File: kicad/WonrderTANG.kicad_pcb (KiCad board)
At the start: 2 copper layers, 101.6 x 90.2 mm, 29 parts, among them CON1 MSX-CONNECTOR, J1 Conn_02x01, J2 AudioJack3, J3 Conn_02x01, Q1 2N3904, U1 SN74LVC245AN, U2 SN74LVC245AN, U3 SN74LVC245AN, U4 SN74LVC245AN, U5 Tang_Nano_20k, U6 SN74LVC245AN

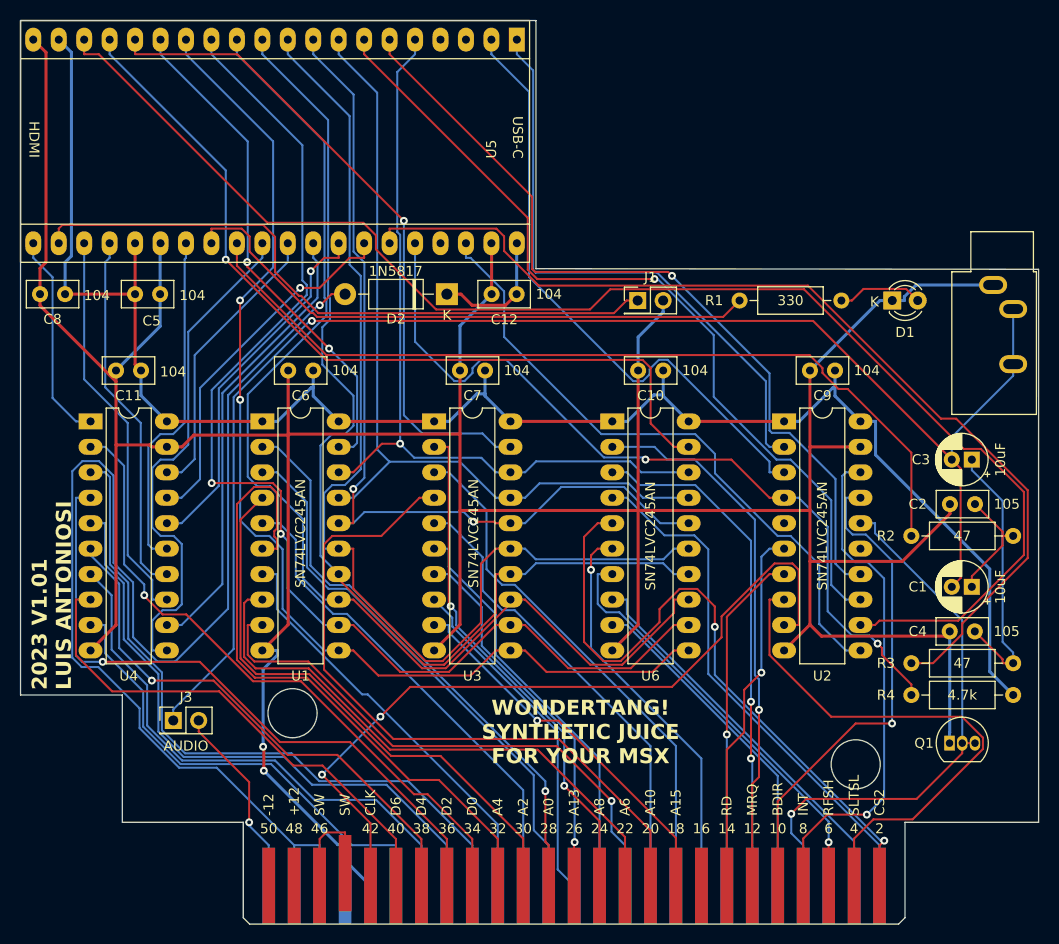
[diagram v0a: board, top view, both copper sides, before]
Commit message: kicad final version 1.01
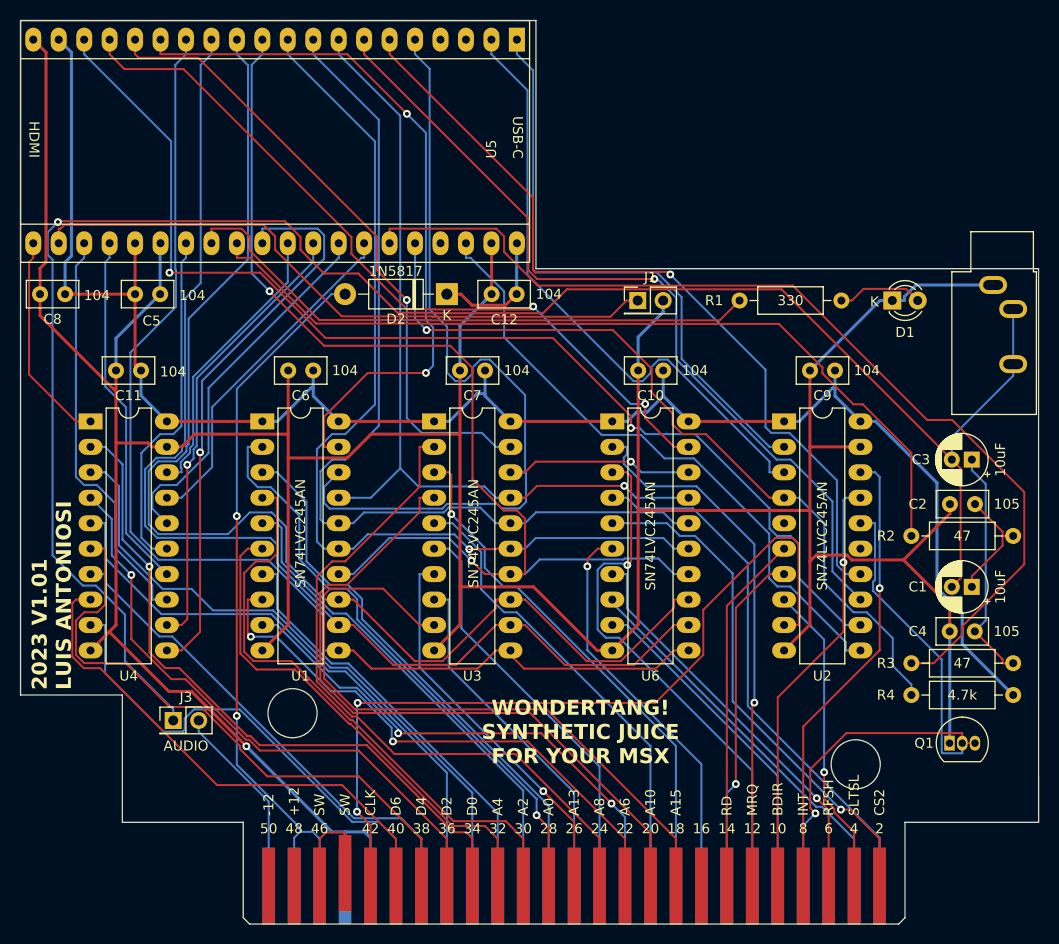
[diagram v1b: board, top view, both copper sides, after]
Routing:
- net Net-(CON1-5V@1): track 132.2 -> 74.1 mm, vias 1 -> 2
- net /AUDIO: track 146.3 -> 188.9 mm
- net A15: track 38.1 -> 67.5 mm, vias 1 -> 0
- net SLTSL_33: track 141.3 -> 114.3 mm, vias 0 -> 2
- net SLTSL: track 54.1 -> 31.5 mm, vias 0 -> 1
- net MSEL0_33: track 50.4 -> 72.2 mm
- net MP0_33: track 79.4 -> 100.9 mm
- net A8: track 51.5 -> 69.3 mm, vias 2 -> 0
- net CS2: track 67.5 -> 51.9 mm, vias 2 -> 1
- net A4: track 65.9 -> 50.3 mm
- net MP3_33: track 108.4 -> 96.4 mm, vias 0 -> 1
- net MP5_33: track 115.2 -> 126.0 mm
- net GND: track 392.0 -> 401.0 mm, vias 2 -> 1
- net MP4_33: track 106.5 -> 113.9 mm, vias 0 -> 2
- net D4: track 53.8 -> 61.0 mm, vias 1 -> 0
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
